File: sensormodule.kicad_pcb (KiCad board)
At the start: 2 copper layers, 20 x 15 mm, 17 parts, among them X1 [Crystal]_32.768KHz

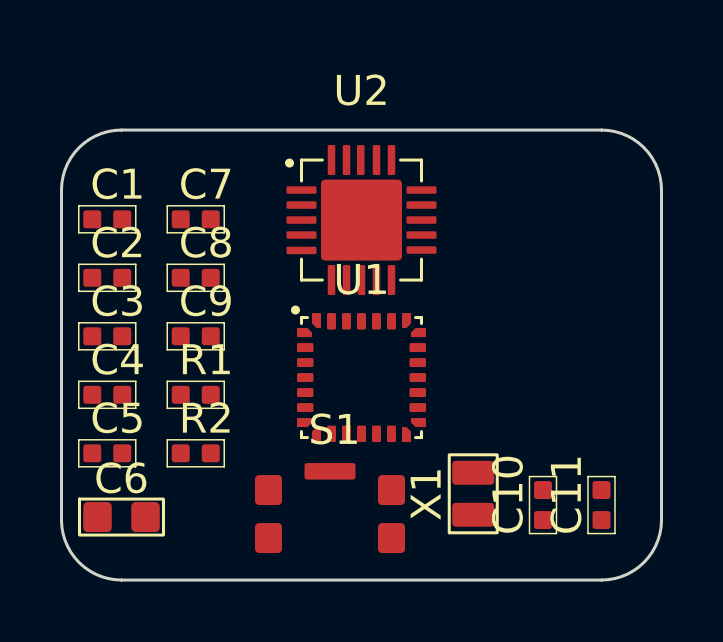
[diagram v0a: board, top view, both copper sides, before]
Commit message: 1
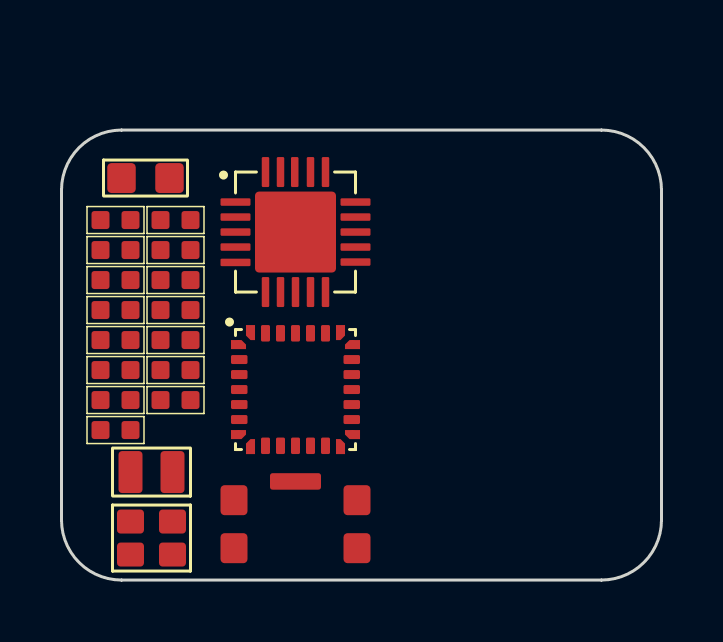
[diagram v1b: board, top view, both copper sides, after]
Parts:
- added C12: 16pF, Kylian:[0402] Capacitor, F.Cu at (87.8, 85.0)
- added C13: 16pF, Kylian:[0402] Capacitor, F.Cu at (89.8, 85.0)
- added R3: 1M, Kylian:[0402] Resistor, F.Cu at (87.8, 86.0)
- added X2: 16MHz, Kylian:[XTAL] 2mmx1.6mm, F.Cu at (89.0, 90.6)
- X1: value [Crystal]_32.768KHz -> 32.768KHz
- moved C11 16.4 mm to (87.8, 87.0), turned to 180 degrees
- moved C10 12.7 mm to (89.8, 86.0), turned to 180 degrees
- moved C6 11.3 mm to (88.8, 78.6)
- moved X1 10.7 mm to (89.0, 88.4), turned to 180 degrees
- moved R2 3.83 mm to (89.8, 84.0)
- moved C5 3.79 mm to (87.8, 84.0)
- moved R1 2.90 mm to (89.8, 83.0)
- moved C4 2.84 mm to (87.8, 83.0)
- moved C8 2.83 mm to (87.8, 81.0)
- moved C1 2.50 mm to (89.8, 81.0)
- moved U1 2.24 mm to (93.8, 85.4)
- moved U2 2.24 mm to (93.8, 80.4)
- moved C9 1.99 mm to (89.8, 82.0)
- moved C2 1.94 mm to (87.8, 80.0)
- moved C3 1.90 mm to (87.8, 82.0)
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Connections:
- U2 pad 10: unconnected-(U2-XC1-Pad10) -> Net-(U2-XC1)
- U2 pad 9: unconnected-(U2-XC2-Pad9) -> Net-(U2-XC2)
